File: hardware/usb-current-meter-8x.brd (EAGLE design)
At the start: 78.5 x 29.2 mm, 40 parts, among them IC3 MEGA48/88/168-AU, IC9 OPA2234U, X7 MC2

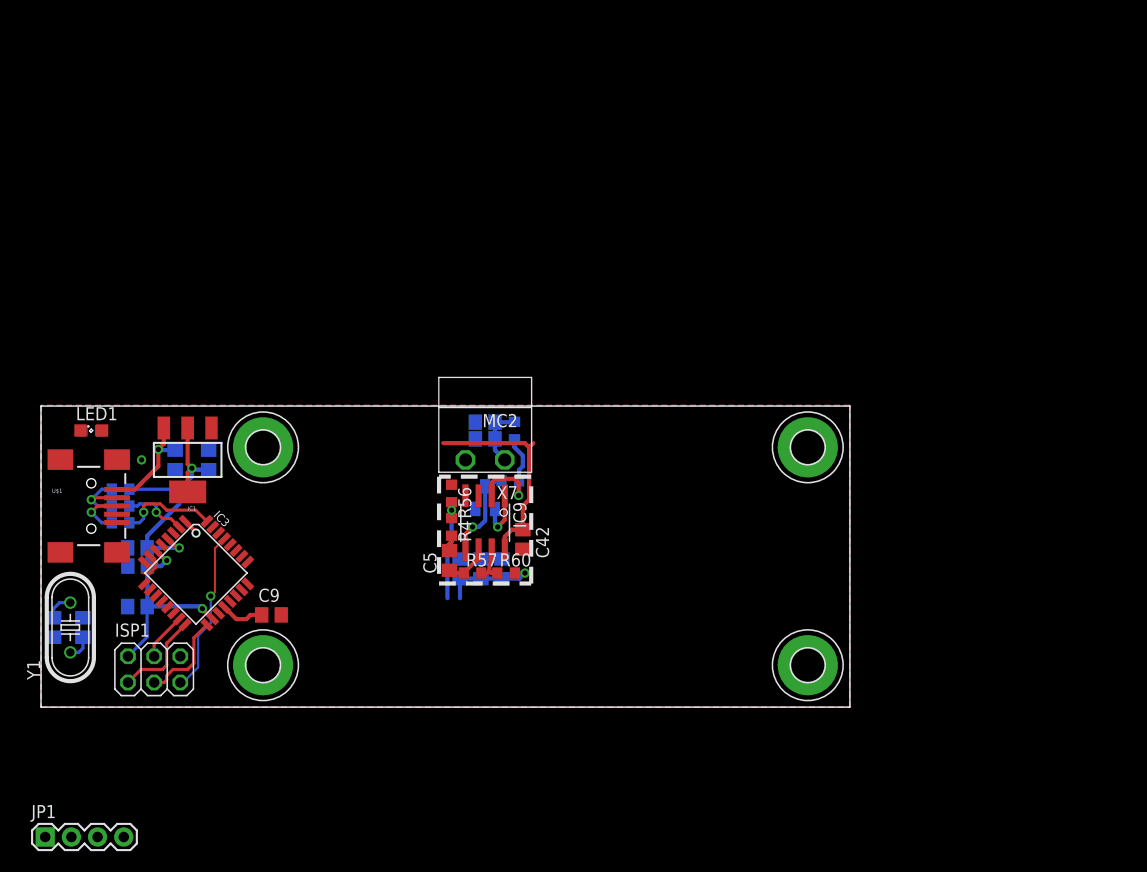
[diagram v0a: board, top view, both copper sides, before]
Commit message: 8x: progress save
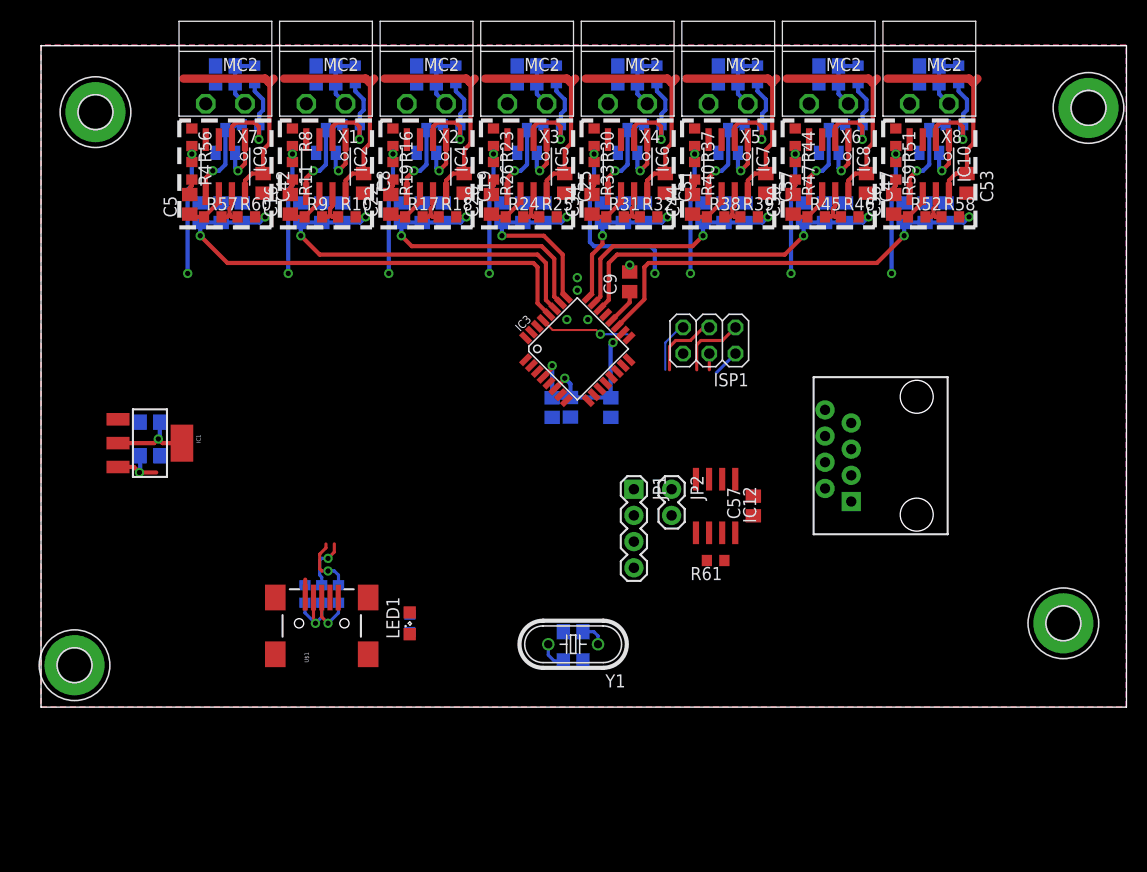
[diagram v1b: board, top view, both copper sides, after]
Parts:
- added C14, C17, C18, C20, C23, C24, C26, C29, C30, C32, C35, C36, C38, C45, C46, C48, C51, C52, C54, C6, C7: 1u, rcl:C0805
- added C15, C19, C21, C25, C27, C31, C33, C37, C39, C47, C49, C53, C55, C8: 100n, rcl:C0805
- added C16, C22, C28, C34, C44, C50, C56: 0, rcl:C0805
- added C57: .1u, rcl:C0805
- added D1, D2, D3, D4, D5, D6, D8: BAT54, diode:SOT23
- added IC10, IC2, IC4, IC5, IC6, IC7, IC8: OPA2234U, burr-brown:SO08
- added IC12: LTC485S, linear-technology:SOIC8
- added JP2: (no value), SparkFun-Connectors:1X02
- added R10, R18, R25, R32, R39, R46, R58: 100k, rcl:R0603
- added R11, R19, R26, R33, R40, R47, R59: Rh, rcl:R0603
- added R12, R20, R27, R34, R41, R48, R5: Rload, rcl:R0805
- added R14, R15, R21, R22, R28, R29, R35, R36, R42, R43, R49, R50, R6, R7: 10k, rcl:R0603
- added R16, R23, R30, R37, R44, R51, R8: Rl, rcl:R0603
- added R17, R24, R31, R38, R45, R52, R9: Rx, rcl:R0603
- added R61: 120, rcl:R0603
- added U3: RJ45-8PTH, SparkFun-Connectors:RJ45-8
- added X1, X2, X3, X4, X5, X6, X8: MC2, con-phoenix-381_l:MC2
- C12, C13, C3, C9: value 100n -> .1u
- C5: value 100n -> 0
- R4: value tbd -> Rh
- R54, R55: value tbd -> 10k
- R56: value tbd -> Rl
- R57: value tbd -> Rx
- moved JP1 66.3 mm to (57.5, 21.1), turned to 270 degrees
- moved ISP1 62.6 mm to (64.8, 35.6), turned to 180 degrees
- moved C10 50.5 mm to (51.6, 4.47), turned to 180 degrees
- moved C12 49.8 mm to (55.3, 29.1), turned to 270 degrees
- moved Y1 48.8 mm to (51.6, 6.10), turned to 180 degrees
- moved C11 47.6 mm to (51.6, 7.32), turned to 0 degrees
- moved C9 47.4 mm to (57.1, 41.2), turned to 90 degrees
- moved C3 44.7 mm to (51.4, 29.1), turned to 270 degrees
- moved IC3 42.9 mm to (52.0, 34.7), turned to 45 degrees
- moved C4 42.8 mm to (17.9, 62.2)
- moved C41 42.8 mm to (15.4, 48.0)
- moved C43 42.8 mm to (19.5, 48.0)
- moved C5 42.8 mm to (14.4, 48.8)
- moved D7 42.8 mm to (17.9, 54.9)
- moved IC9 42.8 mm to (17.9, 52.4)
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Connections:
- removed net MISO: IC3.16, ISP1.1
- removed net MOSI: IC3.15, ISP1.4
- removed net RX: JP1.3
- removed net SCK: IC3.17, ISP1.3
- removed net TX: JP1.2
- new net 485_N: IC12.7, R61.1, U3.2
- new net 485_P: IC12.6, R61.2, U3.1
- new net CH0_IN1: C15.1, R5.2, R6.1, X1.1
- new net CH0_IN2: C21.1, R12.2, R14.1, X2.1
- new net CH0_IN3: C33.1, R27.2, R28.1, X4.1
- new net CH0_IN4: C39.1, R34.2, R35.1, X5.1
- new net CH0_IN5: C55.1, R48.2, R49.1, X8.1
- new net CH0_IN6: C27.1, R20.2, R21.1, X3.1
- new net CH0_IN8: C49.1, R41.2, R42.1, X6.1
- new net N$10: D1.3, IC2.5, R7.2
- new net N$11: C16.1, IC2.6, R9.1
- new net N$12: IC2.7, R10.1, R9.2
- new net N$13: C16.2, R11.2
- new net N$14: IC4.2, R14.2, R15.1
- new net N$15: D2.1, IC4.1
- new net N$16: D2.3, IC4.5, R15.2
- new net N$17: C22.1, IC4.6, R17.1
- new net N$18: IC4.7, R17.2, R18.1
- new net N$19: C22.2, R19.2
- new net N$20: IC6.2, R28.2, R29.1
- new net N$21: D4.1, IC6.1
- new net N$22: D4.3, IC6.5, R29.2
- new net N$23: C34.1, IC6.6, R31.1
- new net N$24: IC6.7, R31.2, R32.1
- new net N$25: C34.2, R33.2
- new net N$26: IC7.2, R35.2, R36.1
- new net N$27: D5.1, IC7.1
- new net N$28: D5.3, IC7.5, R36.2
- new net N$29: C44.1, IC7.6, R38.1
- new net N$30: IC7.7, R38.2, R39.1
- new net N$31: C44.2, R40.2
- new net N$32: IC10.2, R49.2, R50.1
- new net N$33: D8.1, IC10.1
- new net N$34: D8.3, IC10.5, R50.2
- new net N$35: C56.1, IC10.6, R52.1
- new net N$36: IC10.7, R52.2, R58.1
- new net N$42: C56.2, R59.2
- new net N$43: IC5.2, R21.2, R22.1
- new net N$44: D3.1, IC5.1
- new net N$45: D3.3, IC5.5, R22.2
- new net N$46: C28.1, IC5.6, R24.1
- new net N$47: IC5.7, R24.2, R25.1
- new net N$48: C28.2, R26.2
- new net N$49: IC12.1, JP2.2
- new net N$55: IC8.2, R42.2, R43.1
- new net N$56: D6.1, IC8.1
- new net N$57: D6.3, IC8.5, R43.2
- new net N$58: C50.1, IC8.6, R45.1
- new net N$59: IC8.7, R45.2, R46.1
- new net N$60: C50.2, R47.2
- new net N$8: IC2.2, R6.2, R7.1
- new net N$9: D1.1, IC2.1
- new net UART_EN: IC12.2, IC12.3, IC3.1, ISP1.3
- new net UART_RX: IC3.30, JP1.3, JP2.1
- new net UART_TX: IC12.4, IC3.31, JP1.2
- net +5V: now also U3.4, U3.5
- net CH0: now also IC3.28; no longer IC3.23
- net CH0_GAIN: now also IC3.16, ISP1.1; no longer IC3.30
- net CH1: now also C14.1, C6.1, C7.1, IC3.27, R10.2; no longer IC3.24
- net CH1_GAIN: now also IC3.17, ISP1.4, R11.1, R8.2; no longer IC3.31
- net CH2: now also C17.1, C18.1, C20.1, IC3.26, R18.2; no longer IC3.25
- net CH2_GAIN: now also R16.2, R19.1
- net CH3: now also C23.1, C24.1, C26.1, IC3.25, R25.2; no longer IC3.26
- net CH3_GAIN: now also R23.2, R26.1
- net CH4: now also C29.1, C30.1, C32.1, IC3.24, R32.2; no longer IC3.27
- net CH4_GAIN: now also R30.2, R33.1
- net CH5: now also C35.1, C36.1, C38.1, IC3.23, R39.2; no longer IC3.28
- net CH5_GAIN: now also R37.2, R40.1
- net CH6: now also C45.1, C46.1, C48.1, IC3.22, R46.2; no longer IC3.19
- net CH6_GAIN: now also R44.2, R47.1
- net CH7: now also C51.1, C52.1, C54.1, IC3.19, R58.2; no longer IC3.22
- net CH7_GAIN: now also R51.2, R59.1
- net GND: now also C14.2, C15.2, C17.2, C18.2, C19.2, C20.2, C21.2, C23.2, C24.2, C25.2, C26.2, C27.2, C29.2, C30.2, C31.2, C32.2, C33.2, C35.2, C36.2, C37.2, C38.2, C39.2, C45.2, C46.2, C47.2, C48.2, C49.2, C51.2, C52.2, C53.2, C54.2, C55.2, C57.2, C6.2, C7.2, C8.2, IC10.3, IC10.4, IC12.5, IC2.3, IC2.4, IC4.3, IC4.4, IC5.3, IC5.4, IC6.3, IC6.4, IC7.3, IC7.4, IC8.3, IC8.4, R12.1, R16.1, R20.1, R23.1, R27.1, R30.1, R34.1, R37.1, R41.1, R44.1, R48.1, R5.1, R51.1, R8.1, U3.7, U3.8, X1.2, X2.2, X3.2, X4.2, X5.2, X6.2, X8.2
- net LED: now also IC3.15; no longer IC3.1
- net VCC: now also C19.1, C25.1, C31.1, C37.1, C47.1, C53.1, C57.1, C8.1, IC10.8, IC12.8, IC2.8, IC4.8, IC5.8, IC6.8, IC7.8, IC8.8
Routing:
- net VCC: track 69.5 -> 203.0 mm
- net CH7: track 0.00 -> 42.1 mm, vias 0 -> 2
- net CH1: track 0.00 -> 38.5 mm, vias 0 -> 2
- net CH0: track 9.40 -> 47.8 mm, vias 1 -> 2
- net CH6: track 0.00 -> 33.6 mm, vias 0 -> 2
- net CH2: track 0.00 -> 29.1 mm, vias 0 -> 2
- net CH5: track 0.00 -> 24.2 mm, vias 0 -> 2
- net CH3: track 0.00 -> 19.7 mm, vias 0 -> 2
- net CH4_GAIN: track 0.00 -> 19.1 mm, vias 0 -> 2
- net CH4: track 0.00 -> 15.3 mm, vias 0 -> 2
- net CH1_GAIN: track 0.00 -> 14.9 mm, vias 0 -> 2
- net CH7_GAIN: track 0.00 -> 13.3 mm, vias 0 -> 2
- net CH6_GAIN: track 0.00 -> 13.3 mm, vias 0 -> 2
- net CH5_GAIN: track 0.00 -> 13.3 mm, vias 0 -> 2
- net CH3_GAIN: track 0.00 -> 13.3 mm, vias 0 -> 2
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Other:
- board size 78.5 x 29.2 mm -> 105.3 x 64.2 mm

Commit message: 8x: progress save
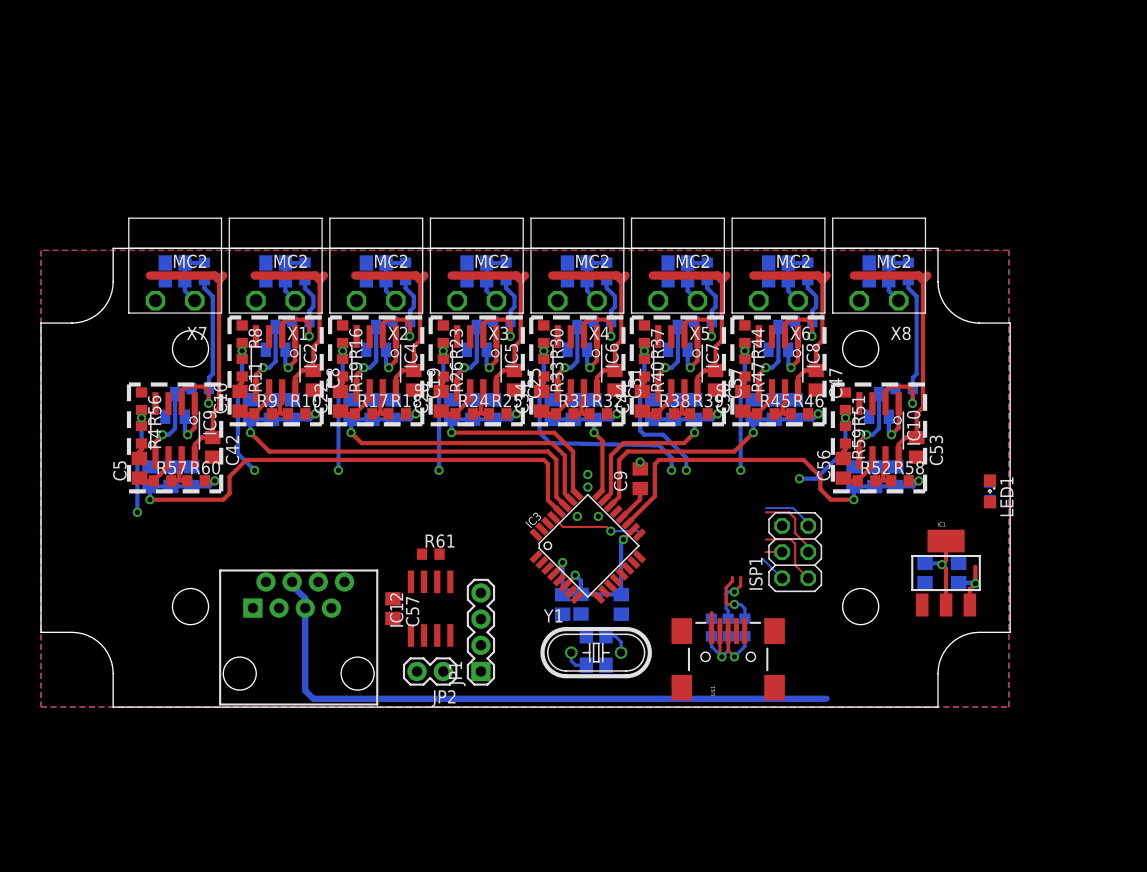
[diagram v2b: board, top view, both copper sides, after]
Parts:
- removed H1, H2, H3, H4: MOUNT-PAD-ROUND3.2, holes:3,2-PAD
- added BOX1: HAMMOND-BOX-XXA, hammond:1591XXA
- moved C2 79.3 mm to (89.0, 13.0), turned to 90 degrees
- moved IC1 78.2 mm to (87.8, 13.0), turned to 0 degrees
- moved C1 76.6 mm to (85.8, 13.0), turned to 270 degrees
- moved U3 63.6 mm to (25.0, 3.25), turned to 0 degrees
- moved LED1 57.7 mm to (92.0, 20.9), turned to 270 degrees
- moved R13 57.7 mm to (92.0, 20.9), turned to 90 degrees
- moved R2 39.6 mm to (66.6, 7.72)
- moved U$1 39.6 mm to (66.6, 4.88)
- moved R1 39.6 mm to (68.3, 7.72)
- moved R3 39.6 mm to (65.0, 7.72)
- moved C57 36.3 mm to (34.1, 9.55), turned to 270 degrees
- moved IC12 29.4 mm to (37.8, 9.55), turned to 0 degrees
- moved JP2 28.3 mm to (39.0, 3.45), turned to 180 degrees
- moved R61 27.6 mm to (37.8, 14.8), turned to 0 degrees
- moved IC10 26.1 mm to (81.3, 26.8)
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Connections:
- net GND: no longer H1.B3,2, H2.B3,2, H3.B3,2, H4.B3,2
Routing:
- net +5V: track 7.32 -> 69.3 mm
- net CH0: track 47.8 -> 55.2 mm
- net N$37: track 11.4 -> 17.9 mm
- net N$32: track 11.4 -> 17.9 mm
- net CH3: track 19.7 -> 25.6 mm
- net CH2: track 29.1 -> 35.0 mm
- net CH1: track 38.5 -> 44.4 mm
- net CH6: track 33.6 -> 27.7 mm
- net CH4_GAIN: track 19.1 -> 24.6 mm
- net CH7: track 42.1 -> 37.4 mm
- net CH7_GAIN: track 13.3 -> 10.2 mm
- net CH5_GAIN: track 13.3 -> 16.2 mm
- net CH0_GAIN: track 20.2 -> 17.8 mm
- net CH5: track 24.2 -> 22.4 mm
- net VCC: track 203.0 -> 202.2 mm
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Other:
- board size 105.3 x 64.2 mm -> 94 x 44.5 mm
